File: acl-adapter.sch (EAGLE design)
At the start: 77 parts, among them IC1 UCC27712, IC2 TL431, IC3 UCC28780, Q1 TLP621-1, T1 COMMON_FILTER-SU10VFC, T2 TRANSFORMAER_FLYBACK-PQ2620

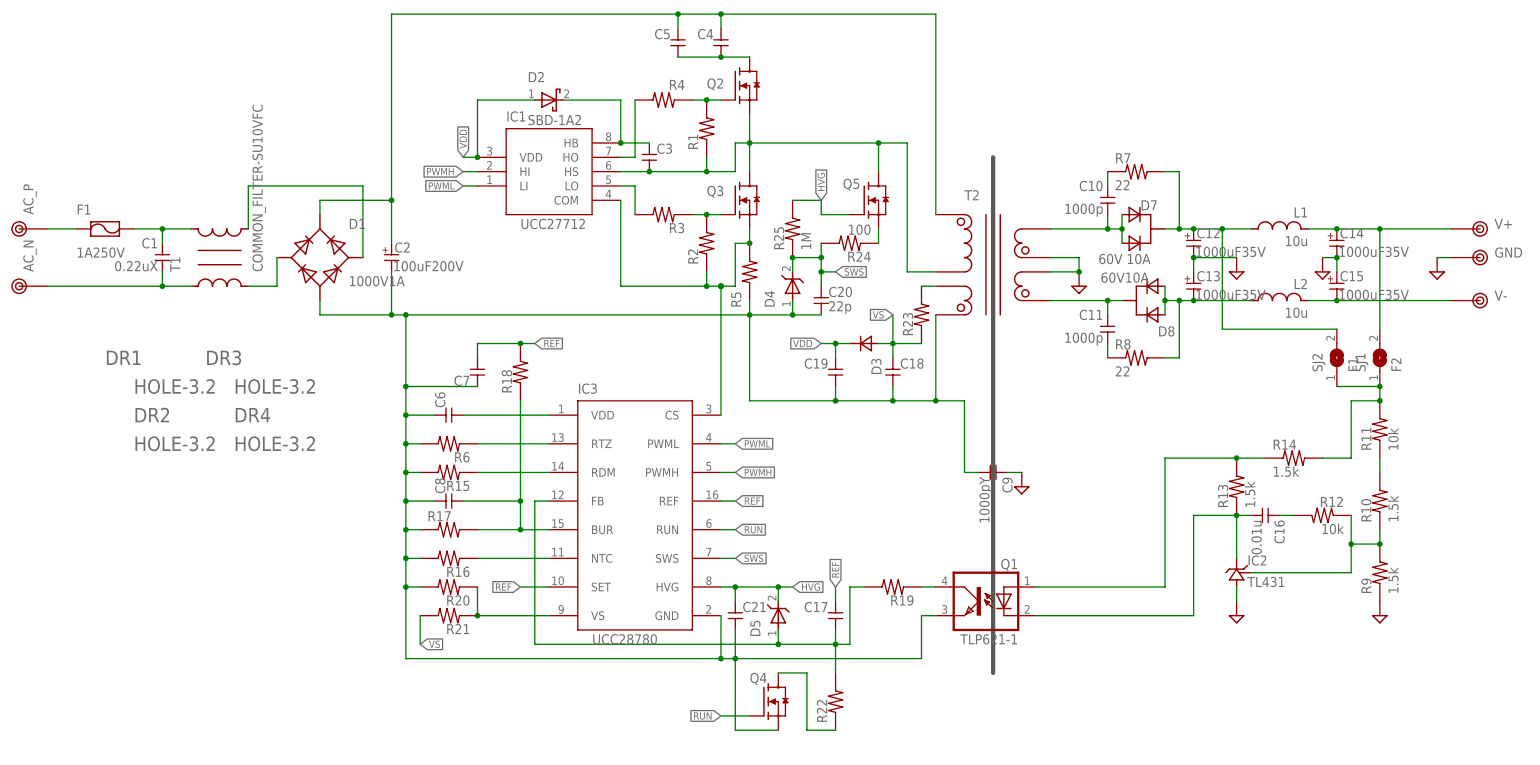
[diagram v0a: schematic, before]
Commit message: 回路図できた
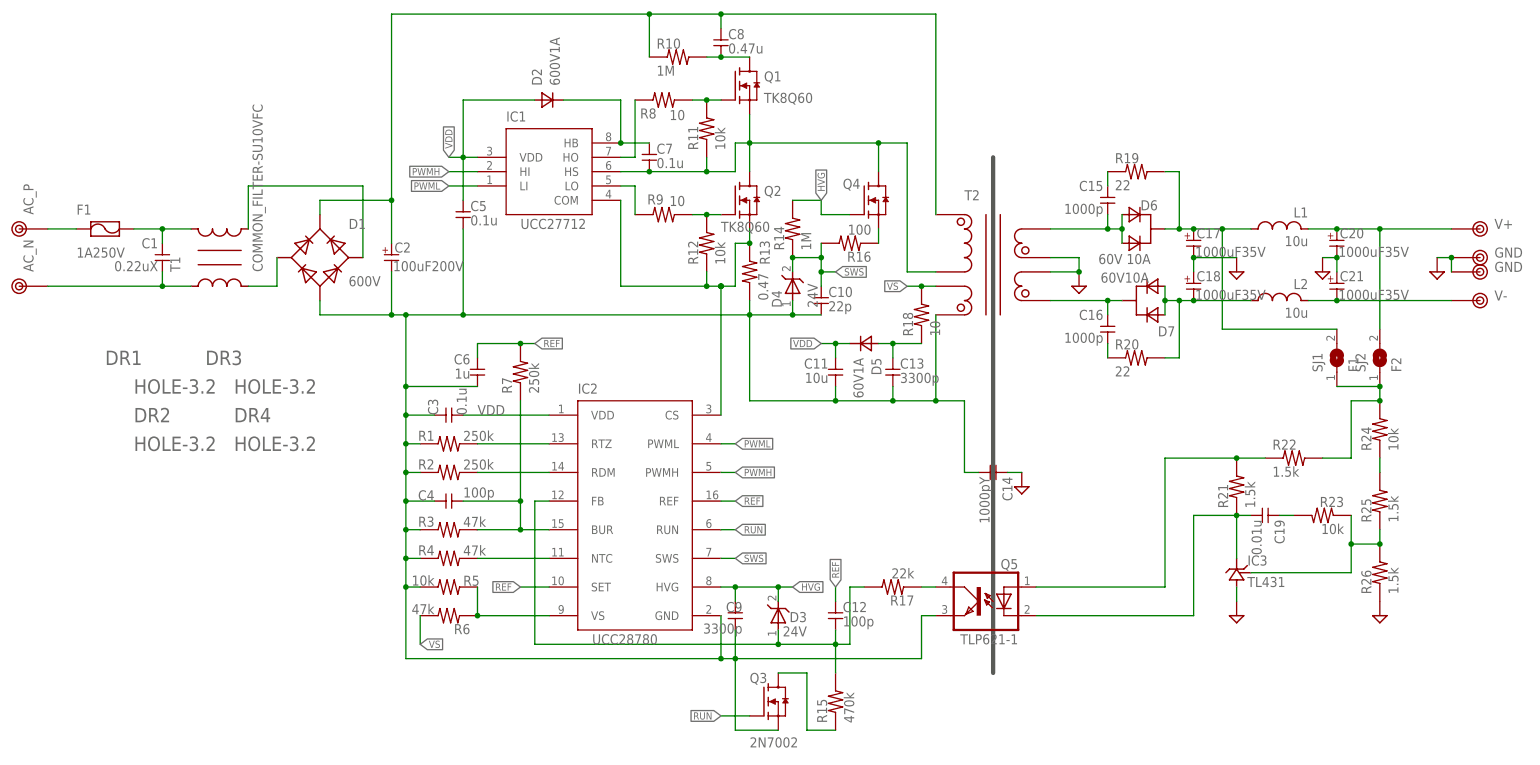
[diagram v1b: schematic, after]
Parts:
- removed D8: 60V10A, my_rcl:DIODE2
- added D6: 60V 10A, my_rcl:DIODE2
- added R26: 1.5k, my_rcl:R-1608
- added TP6: GND, my_connector:TESTPIN-BIG
- C10: value 1000p -> 22p
- C11: value 1000p -> 10u; device my_rcl:C-1608 -> my_rcl:C-2012
- C12: value 1000uF35V -> 100p; device my_rcl:CPOLE5-13 -> my_rcl:C-1608
- C13: value 1000uF35V -> 3300p; device my_rcl:CPOLE5-13 -> my_rcl:C-1608
- C14: value 1000uF35V -> 1000pY; device my_rcl:CPOLE5-10 -> my_rcl:C-Y
- C15: value 1000uF35V -> 1000p; device my_rcl:CPOLE5-10 -> my_rcl:C-1608
- C16: value 0.01u -> 1000p
- C17, C18, C21: value (none) -> 1000uF35V; device my_rcl:C-1608 -> my_rcl:CPOLE5-10
- C19: value (none) -> 0.01u; device my_rcl:C-2012 -> my_rcl:C-1608
- C20: value 22p -> 1000uF35V; device my_rcl:C-1608 -> my_rcl:CPOLE5-10
- C3: value (none) -> 0.1u; device my_rcl:C-2012 -> my_rcl:C-1608
- C4: value (none) -> 100p; device my_rcl:C-5 -> my_rcl:C-2012
- C5: value (none) -> 0.1u; device my_rcl:C-5 -> my_rcl:C-1608
- C6: value (none) -> 1u
- C7: value (none) -> 0.1u
- C8: value (none) -> 0.47u; device my_rcl:C-2012 -> my_rcl:C-7.5
- C9: value 1000pY -> 3300p; device my_rcl:C-Y -> my_rcl:C-1608
- D1: value 1000V1A -> 600V
- D2: value SBD-1A2 -> 600V1A; device my_rcl:SBD-1A2 -> my_rcl:DIODE-2
- D3: value (none) -> 24V; device my_rcl:DIODE-2 -> my_rcl:ZENER-SMD
- D4: value (none) -> 24V; device my_rcl:ZENER -> my_rcl:ZENER-SMD
- D5: value (none) -> 60V1A; device my_rcl:ZENER -> my_rcl:DIODE-2
- D7: value 60V 10A -> 60V10A
- IC2: value TL431 -> UCC28780; device my_ic:TL431 -> my_ic:UCC28780
- IC3: value UCC28780 -> TL431; device my_ic:UCC28780 -> my_ic:TL431
- Q1: value TLP621-1 -> TK8Q60; device my_ic:TLP621-1 -> my_ic:NMOS
- Q2: value (none) -> TK8Q60
- Q3: value (none) -> 2N7002; device my_ic:NMOS -> my_ic:NMOS-SMD
- Q5: value (none) -> TLP621-1; device my_ic:NMOS-SMD -> my_ic:TLP621-1
- R1, R2: value (none) -> 250k
- R10: value 1.5k -> 1M; device my_rcl:R-1608 -> my_rcl:R-7.5
- R13: value 1.5k -> 0.47; device my_rcl:R-1608 -> my_rcl:R-10
- R14: value 1.5k -> 1M
- R15: value (none) -> 470k; device my_rcl:R-2.5 -> my_rcl:R-1608
- R16: value (none) -> 100; device my_rcl:R-2.5 -> my_rcl:R-1608
- R17: value (none) -> 22k; device my_rcl:R-2.5 -> my_rcl:R-1608
- R18: value (none) -> 10; device my_rcl:R-2.5 -> my_rcl:R-1608
- R19: value (none) -> 22
- R20: value (none) -> 22; device my_rcl:R-1608 -> my_rcl:R-2.5
- R21: value (none) -> 1.5k; device my_rcl:R-2.5 -> my_rcl:R-1608
- R22: value (none) -> 1.5k
- R23: value (none) -> 10k; device my_rcl:R-2.5 -> my_rcl:R-1608
- R24: value 100 -> 10k
- R25: value 1M -> 1.5k
- R3, R4: value (none) -> 47k
- R5: value (none) -> 10k; device my_rcl:R-7.5 -> my_rcl:R-1608
- R6: value (none) -> 47k; device my_rcl:R-2.5 -> my_rcl:R-1608
- R7: value 22 -> 250k; device my_rcl:R-2.5 -> my_rcl:R-1608
- R8: value 22 -> 10; device my_rcl:R-2.5 -> my_rcl:R-1608
- R9: value 1.5k -> 10
- SJ1: value F2 -> F1
- SJ2: value F1 -> F2
- T2: value TRANSFORMAER_FLYBACK-PQ2620 -> TRANSFORMAER_FLYBACK-PQ2620-ACF; device my_rcl:TRANSFORMAER_FLYBACK-PQ2620 -> my_rcl:TRANSFORMAER_FLYBACK-PQ2620-ACF
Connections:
- removed net N$30: R23.2, T2.L2_N
- removed net N$31: C6.2, IC3.VDD
- removed net N$41: C17.2, D5.A, IC3.FB, R19.2, R22.2
- new net FB: C12.2, D3.A, IC2.FB, R15.2, R17.2
- new net N$19: C13.1, D5.A, R18.1
- net GND: now also C14.1, C17.2, C18.1, C20.2, C21.1, IC3.GND, R26.1, TP6.1; no longer C12.2, C13.1, C14.2, C15.1, C9.1, IC2.GND, R9.1
- net HVG: now also C9.1, D3.C, IC2.HVG, Q4.G, R14.2; no longer C21.1, D5.C, IC3.HVG, Q5.G, R25.2
- net N$10: now also C7.1; no longer C3.1
- net N$11: now also R8.2; no longer R4.2
- net N$12: now also Q1.G, R11.2, R8.1; no longer Q2.G, R1.2, R4.1
- net N$13: now also C8.2, Q1.D, R10.2; no longer C4.2, C5.2, Q2.D
- net N$14: now also R9.2; no longer R3.2
- net N$15: now also IC2.CS, Q2.S, R12.1, R13.2; no longer IC3.CS, Q3.S, R2.1, R5.2
- net N$16: now also Q4.S, R16.1; no longer Q5.S, R24.1
- net N$17: now also C15.2, D6.A1, D6.A2; no longer C10.2, D7.A1, D7.A2
- net N$18: now also C16.1, D7.K; no longer C11.1, D8.K
- net N$20: now also IC2.RTZ, R1.1; no longer IC3.RTZ, R6.1
- net N$21: now also IC2.RDM, R2.1; no longer IC3.RDM, R15.1
- net N$22: now also C16.2, R20.1; no longer C11.2, R8.1
- net N$23: now also C18.2, D7.A1, D7.A2, R20.2; no longer C13.2, D8.A1, D8.A2, R8.2
- net N$24: now also IC2.NTC, R4.1; no longer IC3.NTC, R16.1
- net N$25: now also R24.1, R25.2; no longer R10.2, R11.1
- net N$26: now also IC3.REF, R23.1, R25.1, R26.2; no longer IC2.REF, R10.1, R12.1, R9.2
- net N$27: now also C19.1, R23.2; no longer C16.1, R12.2
- net N$28: now also C19.2, IC3.OUT, Q5.C, R21.1; no longer C16.2, IC2.OUT, Q1.C, R13.1
- net N$29: now also Q5.A, R21.2, R22.1; no longer Q1.A, R13.2, R14.1
- net N$32: now also C4.2, IC2.BUR, R3.2, R7.1; no longer C8.2, IC3.BUR, R17.2, R18.1
- net N$34: now also Q3.D, R15.1; no longer Q4.D, R22.1
- net N$35: now also Q5.COL, R17.1; no longer Q1.COL, R19.1
- net N$36: now also IC2.VS, R5.1, R6.1; no longer IC3.VS, R20.1, R21.1
- net N$40: now also C7.2, Q1.S, Q2.D, Q4.D, R11.1; no longer C3.2, Q2.S, Q3.D, Q5.D, R1.1
- net N$6: now also C17.1, D6.K, R19.2, SJ1.2; no longer C12.1, D7.K, R7.2, SJ2.2
- net N$7: now also Q2.G, R12.2, R9.1; no longer Q3.G, R2.2, R3.1
- net N$8: now also C15.1, R19.1; no longer C10.1, R7.1
- net N$9: now also R22.2, R24.2; no longer R11.2, R14.2
- net PGND: now also C10.2, C11.2, C13.2, C14.2, C3.1, C4.1, C5.2, IC2.GND, Q3.S, Q5.EMIT, R1.2, R13.1, R2.2, R3.1, R4.2, R5.2; no longer C18.2, C19.2, C20.2, C21.2, C7.1, C8.1, IC3.GND, Q1.EMIT, Q4.S, R15.2, R16.2, R17.1, R20.2, R5.1, R6.2
- net PWMH: now also IC2.PWMH; no longer IC3.PWMH
- net PWML: now also IC2.PWML; no longer IC3.PWML
- net REF: now also C12.1, C6.2, IC2.REF, IC2.SET, R7.2; no longer C17.1, C7.2, IC3.REF, IC3.SET, R18.2
- net RUN: now also IC2.RUN, Q3.G; no longer IC3.RUN, Q4.G
- net SWS: now also C10.1, IC2.SWS, R14.1, R16.2; no longer C20.1, IC3.SWS, R24.2, R25.1
- net V+: now also C20.1, SJ2.2; no longer C14.1, SJ1.2
- net V-: now also C21.2; no longer C15.2
- net VDD: now also C11.1, C3.2, C5.1, D5.K, IC2.VDD; no longer C19.1, D3.K
- net VP: now also C8.1, R10.1; no longer C4.1, C5.1
- net VS: now also R18.2, R6.2, T2.L2_N; no longer C18.1, D3.A, R21.2, R23.1
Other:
- moved on the sheet: C10, C11, C16, C19, C3, C4, C5, C6, C7, C8, C9, D7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
